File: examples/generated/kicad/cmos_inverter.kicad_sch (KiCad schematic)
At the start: 4 parts

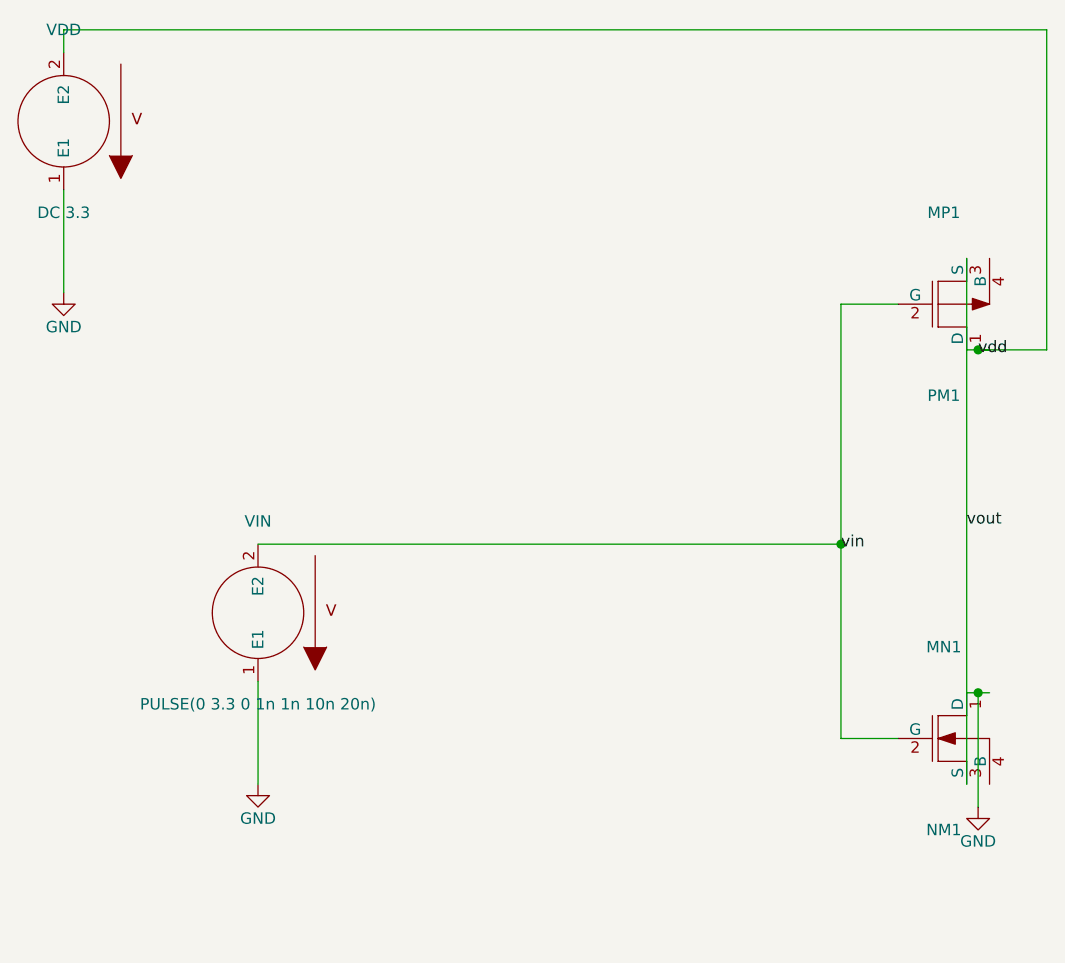
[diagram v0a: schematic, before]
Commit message: Attempt again to fix cmos topology.
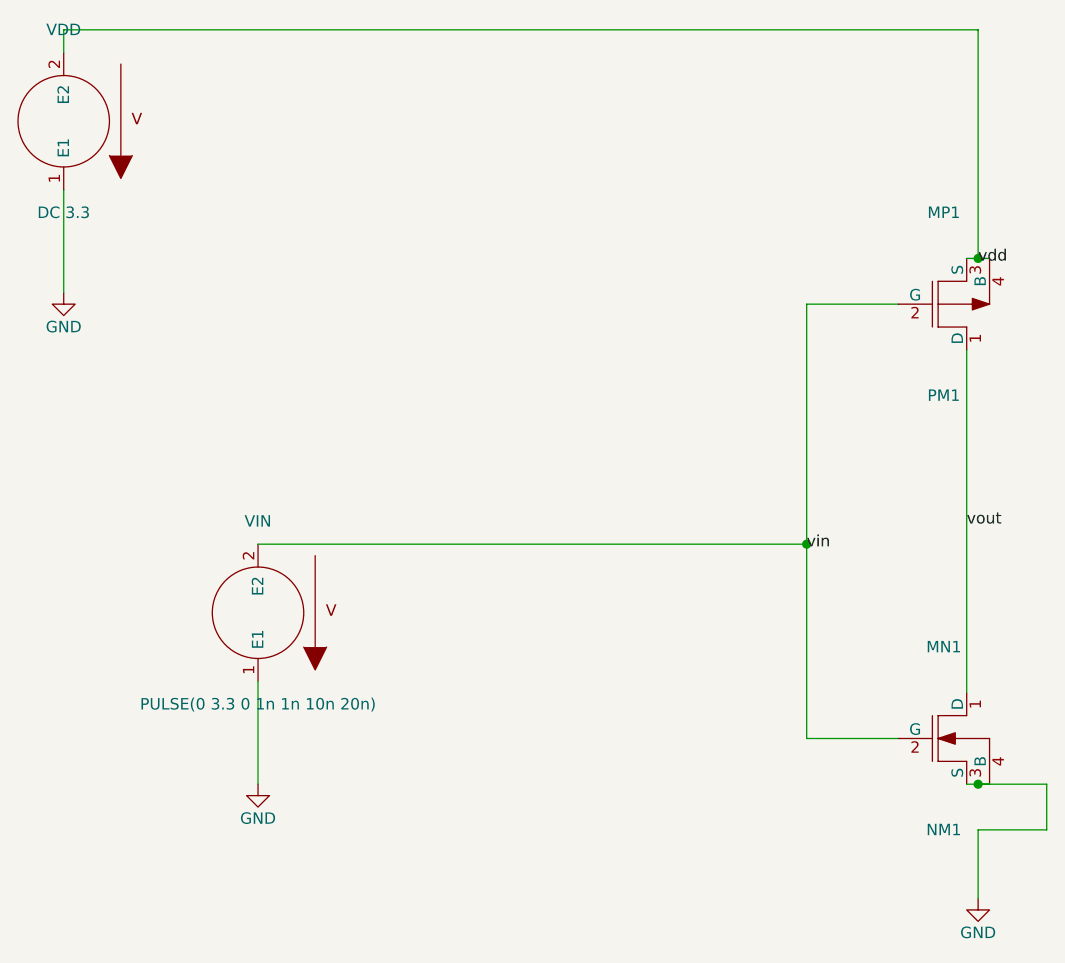
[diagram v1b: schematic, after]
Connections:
- net GND: now also MN1.3 (S), MN1.4 (B); no longer MN1.1 (D)
- net vdd: now also MP1.3 (S), MP1.4 (B); no longer MP1.1 (D)
- net vout: now also MN1.1 (D), MP1.1 (D); no longer MN1.3 (S), MP1.3 (S)
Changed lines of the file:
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@@
     )
   )
-  (symbol (lib_id "GND") (at 163.83 144.78 0) (unit 1)
+  (symbol (lib_id "GND") (at 163.83 154.94 0) (unit 1)
     (in_bom yes) (on_board yes)
-    (property "Reference" "#PWR0003" (at 163.83 140.97 0)
+    (property "Reference" "#PWR0003" (at 163.83 151.13 0)
       (effects (font (size 1.27 1.27)) hide)
     )
-    (property "Value" "GND" (at 163.83 148.59 0)
+    (property "Value" "GND" (at 163.83 158.75 0)
       (effects (font (size 1.27 1.27)))
     )
@@
     )
   )
-  (label "vin" (at 148.59 115.57 0)
+  (label "vin" (at 144.78 115.57 0)
     (effects (font (size 1.27 1.27)))
   )
-  (label "vdd" (at 163.83 93.98 0)
+  (label "vdd" (at 163.83 83.82 0)
     (effects (font (size 1.27 1.27)))
   )
@@
     (stroke (width 0) (type solid) (color 0 0 0 0))
   )
-  (wire (pts (xy 148.59 88.90) (xy 148.59 137.16))
+  (wire (pts (xy 144.78 88.90) (xy 144.78 137.16))
     (stroke (width 0) (type solid) (color 0 0 0 0))
   )
-  (wire (pts (xy 83.82 115.57) (xy 148.59 115.57))
+  (wire (pts (xy 83.82 115.57) (xy 144.78 115.57))
     (stroke (width 0) (type solid) (color 0 0 0 0))
   )
-  (wire (pts (xy 154.94 88.90) (xy 148.59 88.90))
+  (wire (pts (xy 154.94 88.90) (xy 144.78 88.90))
     (stroke (width 0) (type solid) (color 0 0 0 0))
   )
-  (wire (pts (xy 154.94 137.16) (xy 148.59 137.16))
+  (wire (pts (xy 154.94 137.16) (xy 144.78 137.16))
     (stroke (width 0) (type solid) (color 0 0 0 0))
   )
@@
     (stroke (width 0) (type solid) (color 0 0 0 0))
   )
-  (wire (pts (xy 62.23 58.42) (xy 171.45 58.42))
+  (wire (pts (xy 62.23 58.42) (xy 163.83 58.42))
     (stroke (width 0) (type solid) (color 0 0 0 0))
   )
-  (wire (pts (xy 171.45 58.42) (xy 171.45 93.98))
+  (wire (pts (xy 163.83 58.42) (xy 163.83 83.82))
     (stroke (width 0) (type solid) (color 0 0 0 0))
   )
-  (wire (pts (xy 171.45 93.98) (xy 163.83 93.98))
+  (wire (pts (xy 162.56 83.82) (xy 163.83 83.82))
     (stroke (width 0) (type solid) (color 0 0 0 0))
   )
-  (wire (pts (xy 162.56 93.98) (xy 163.83 93.98))
+  (wire (pts (xy 165.10 83.82) (xy 163.83 83.82))
     (stroke (width 0) (type solid) (color 0 0 0 0))
   )
-  (wire (pts (xy 165.10 93.98) (xy 163.83 93.98))
+  (wire (pts (xy 162.56 93.98) (xy 162.56 132.08))
     (stroke (width 0) (type solid) (color 0 0 0 0))
   )
-  (wire (pts (xy 162.56 83.82) (xy 162.56 142.24))
+  (wire (pts (xy 162.56 142.24) (xy 163.83 142.24))
     (stroke (width 0) (type solid) (color 0 0 0 0))
   )
-  (wire (pts (xy 162.56 132.08) (xy 163.83 132.08))
+  (wire (pts (xy 165.10 142.24) (xy 163.83 142.24))
     (stroke (width 0) (type solid) (color 0 0 0 0))
   )
-  (wire (pts (xy 165.10 132.08) (xy 163.83 132.08))
+  (wire (pts (xy 163.83 154.94) (xy 163.83 147.32))
     (stroke (width 0) (type solid) (color 0 0 0 0))
   )
-  (wire (pts (xy 163.83 144.78) (xy 163.83 132.08))
+  (wire (pts (xy 163.83 147.32) (xy 171.45 147.32))
     (stroke (width 0) (type solid) (color 0 0 0 0))
   )
-  (junction (at 148.59 115.57) (diameter 1.016) (color 0 0 0 0))
-  (junction (at 163.83 93.98) (diameter 1.016) (color 0 0 0 0))
-  (junction (at 163.83 132.08) (diameter 1.016) (color 0 0 0 0))
+  (wire (pts (xy 171.45 147.32) (xy 171.45 142.24))
+    (stroke (width 0) (type solid) (color 0 0 0 0))
+  )
+  (wire (pts (xy 171.45 142.24) (xy 163.83 142.24))
+    (stroke (width 0) (type solid) (color 0 0 0 0))
+  )
+  (junction (at 144.78 115.57) (diameter 1.016) (color 0 0 0 0))
+  (junction (at 163.83 83.82) (diameter 1.016) (color 0 0 0 0))
+  (junction (at 163.83 142.24) (diameter 1.016) (color 0 0 0 0))
   (sheet_instances
     (path "/" (page "1"))
